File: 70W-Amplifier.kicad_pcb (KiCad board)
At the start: 2 copper layers, 170.9 x 81 mm, 35 parts, among them J1 RF_OUT, J2 RF_IN, J3 LPF_IN, J4 LPF_OUT, J5 13.8V Input, J6 PTT, K1 G5V-2, Q1 2N3906-SMD, Q2 IRF530, Q3 IRF530, T1 BN-43-202 1T:2T, T2 Ferrite 1T:3T, U1 L7805

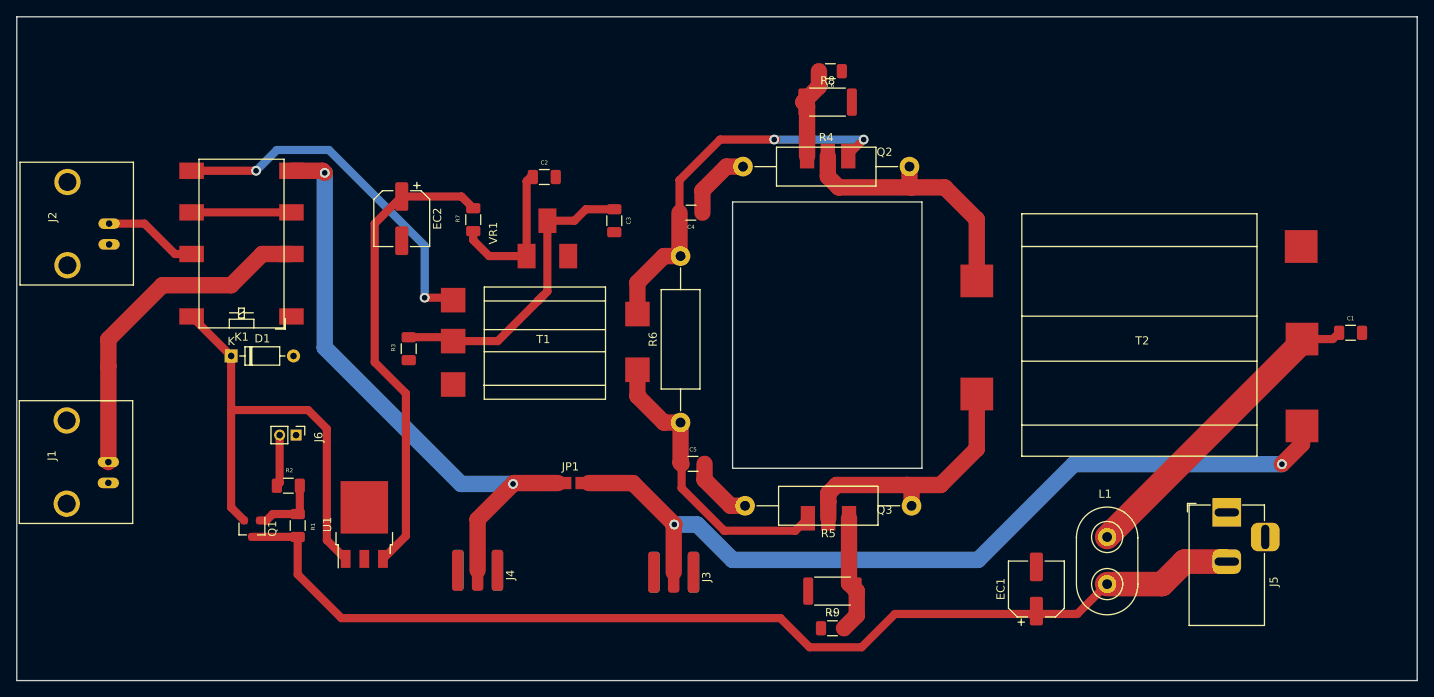
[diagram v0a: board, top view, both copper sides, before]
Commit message: finished
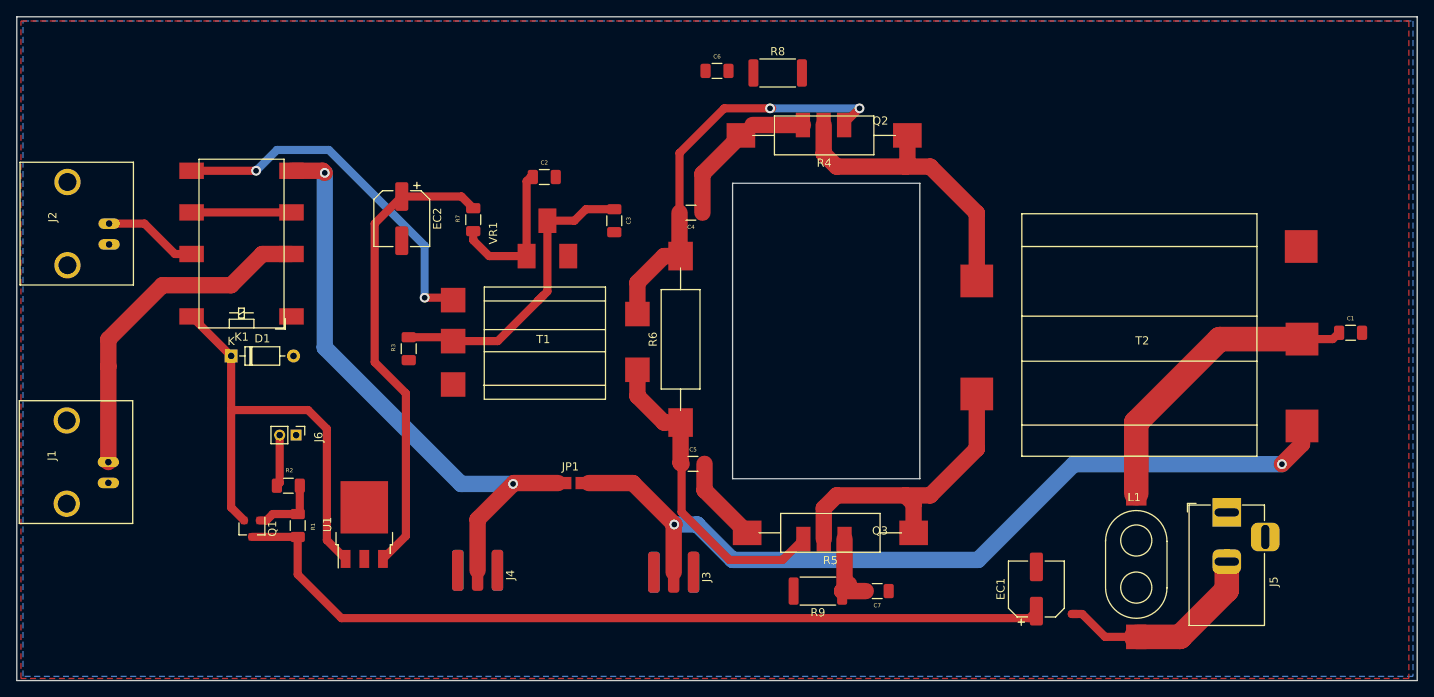
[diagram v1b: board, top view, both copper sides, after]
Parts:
- L1: footprint Xenir:BN-43-202-Vertical -> Xenir:BN-43-202-Vertical-SMD
- R4, R5, R6: footprint Resistor_THT:R_Axial_DIN0414_L11.9mm_D4.5mm_P20.32mm_Horizontal -> Xenir:LargeResistorSurfaceMount
- moved C6 14.6 mm to (161.7, 47.5), turned to 0 degrees
- moved R8 7.06 mm to (169.1, 50.0)
- moved C7 5.46 mm to (181.2, 115.5), turned to 180 degrees
- moved Q2 3.84 mm to (174.5, 62.3)
- moved R4 3.82 mm to (184.9, 57.7)
- moved L1 3.58 mm to (212.9, 117.9)
- moved R5 3.31 mm to (185.7, 106.2)
- moved Q3 2.60 mm to (174.9, 101.0)
- moved R9 1.78 mm to (174.0, 113.3)
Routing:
- net Net-(C6-Pad2): track 11.4 -> 6.15 mm
- net /Q2Drain: track 33.0 -> 37.4 mm
- net /Q3Drain: track 32.9 -> 37.1 mm
- net Net-(C7-Pad2): track 14.5 -> 10.5 mm
- net Net-(C5-Pad1): track 36.1 -> 39.1 mm
- net Net-(C4-Pad2): track 47.4 -> 50.4 mm
- net Net-(C5-Pad2): track 8.21 -> 10.6 mm
- net Net-(C4-Pad1): track 8.86 -> 11.1 mm
- net +12V: track 131.6 -> 129.5 mm
- net Net-(C1-Pad1): track 38.9 -> 38.3 mm
- added copper zone on B.Cu, net GND
- added copper zone on F.Cu, net GND
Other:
- outline, holes or cut-outs redrawn

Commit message: Update 70W-Amplifier.kicad_pcb
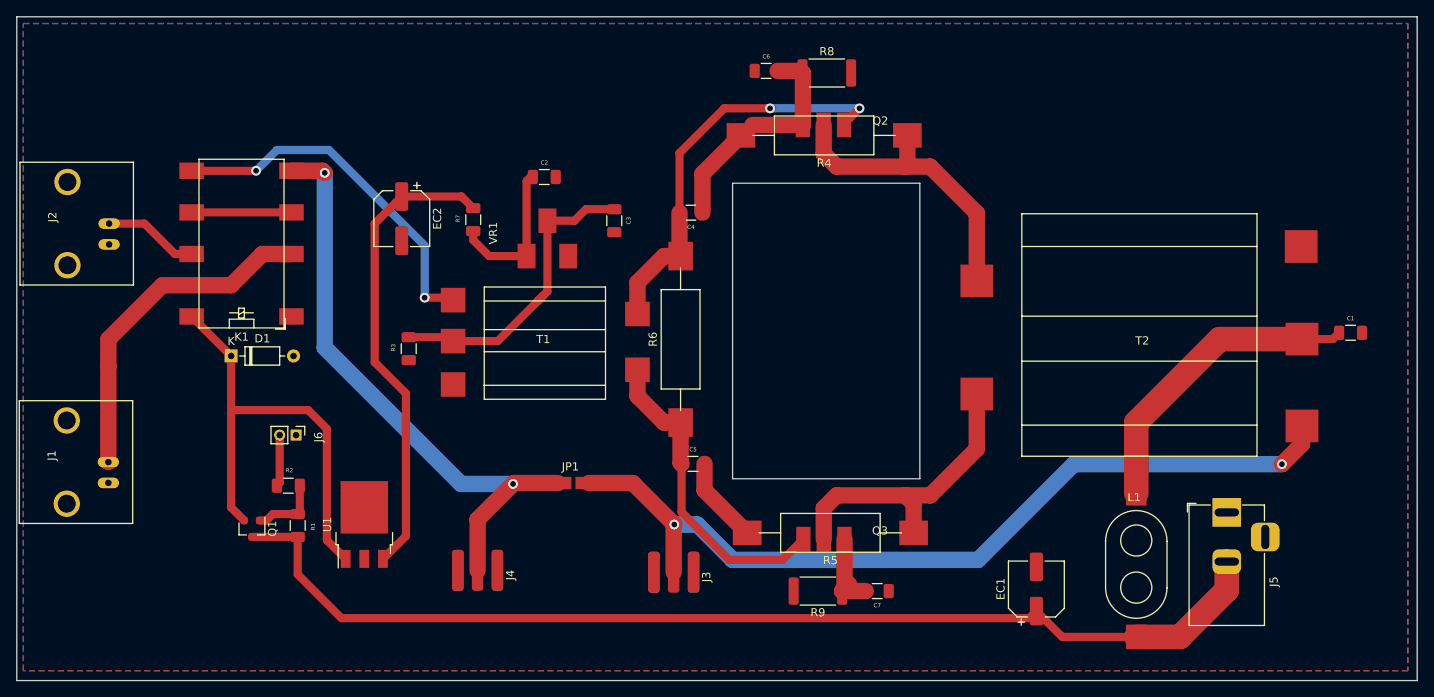
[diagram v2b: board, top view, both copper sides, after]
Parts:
- moved C6 6.00 mm to (167.7, 47.5)
- moved R8 6.00 mm to (175.1, 50.0)
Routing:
- net Net-(C6-Pad2): track 6.15 -> 15.7 mm
- net +12V: track 129.5 -> 133.3 mm
